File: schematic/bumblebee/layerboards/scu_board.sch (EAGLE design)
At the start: 19 parts, among them P5 B4B-EH-A, P7 B3B-EH-A, X1 332-02, X2 332-02, X3 332-02, X4 332-02, X5 332-02

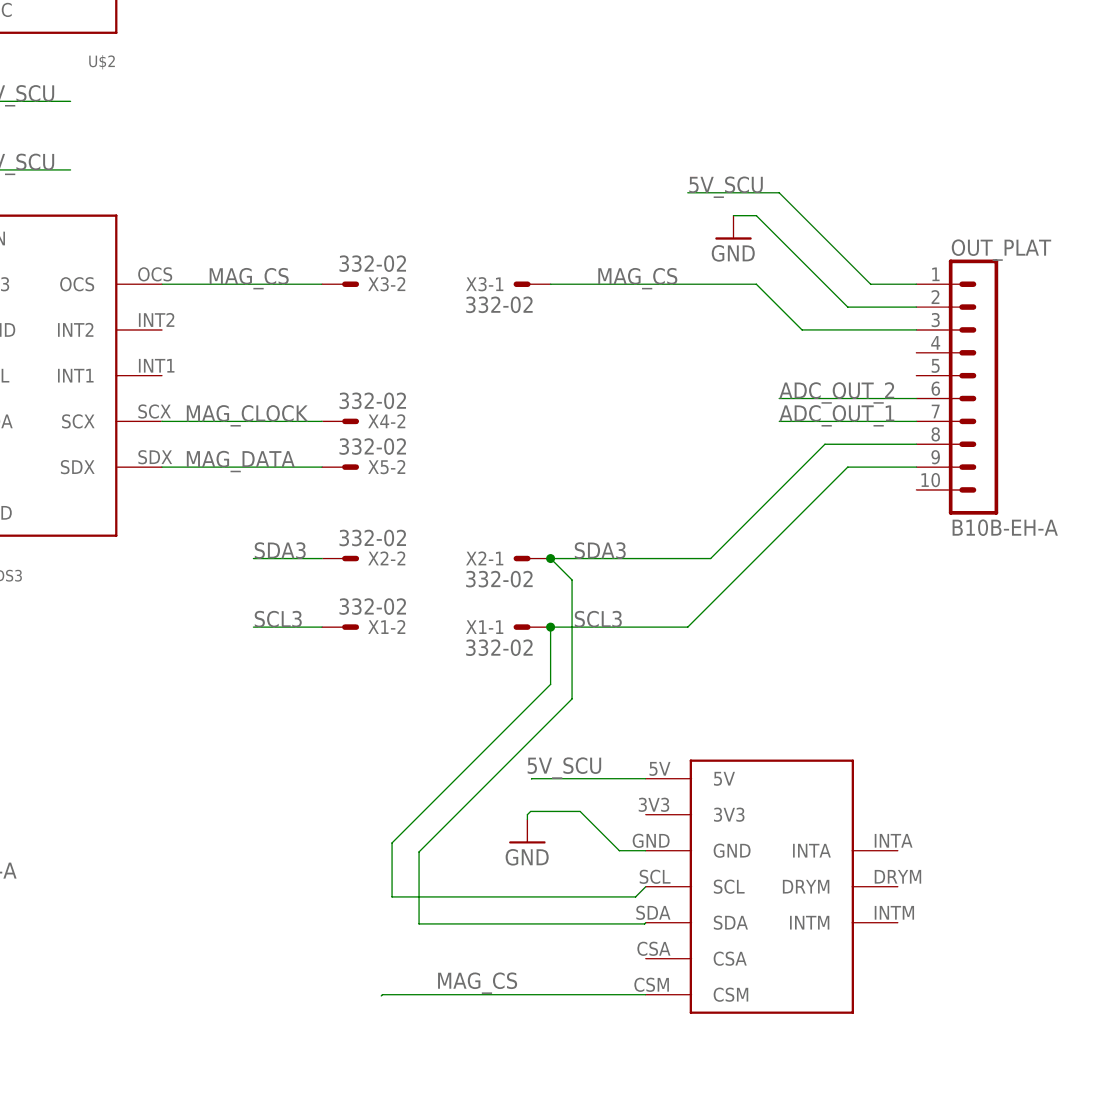
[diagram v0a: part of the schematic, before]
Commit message: Готова SCU и поправил lsm303c в либе
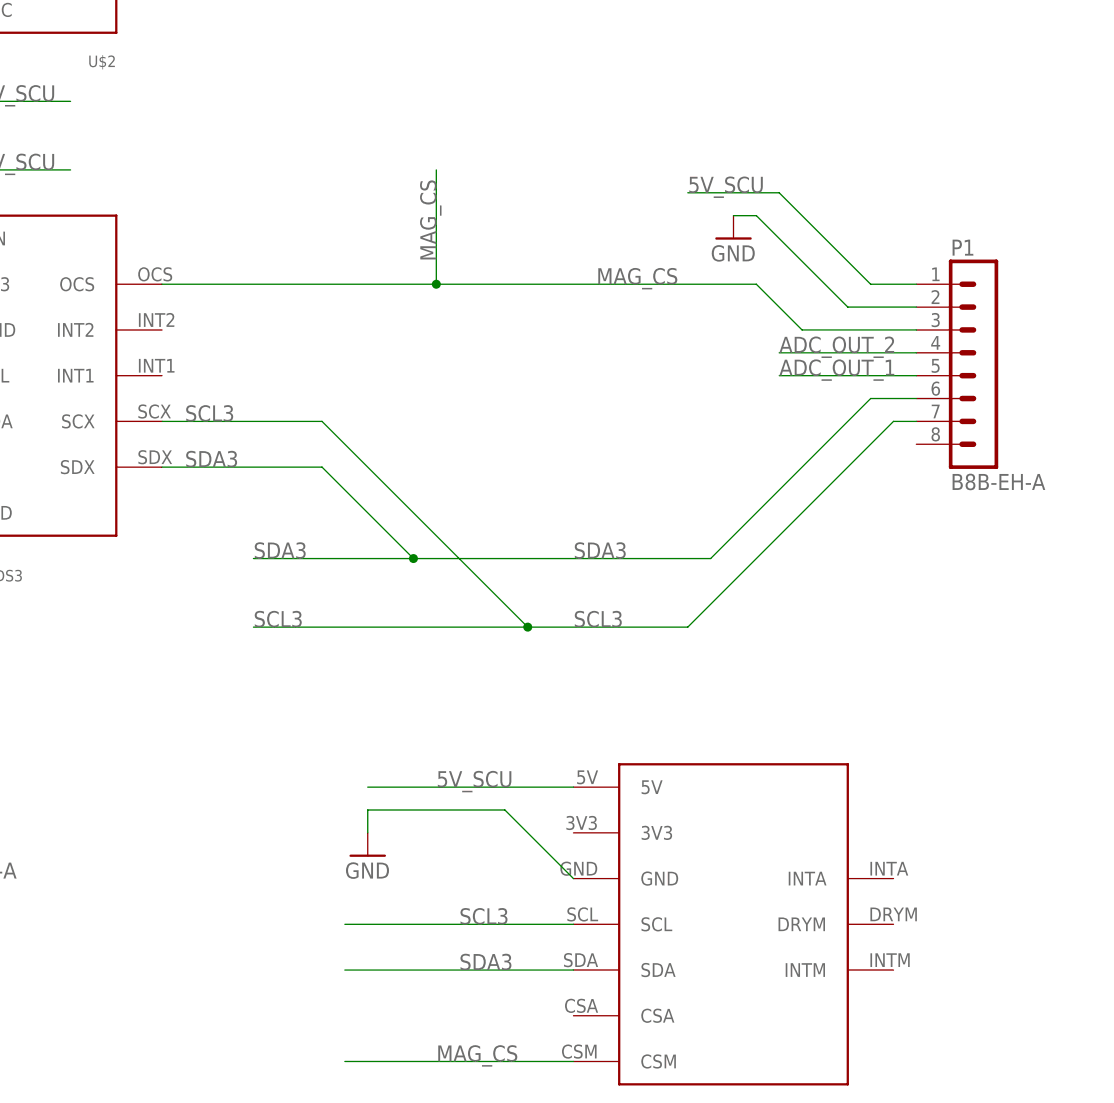
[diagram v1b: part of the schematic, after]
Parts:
- removed OUT_PLAT: B10B-EH-A, con-jst-eh:B10B-EH-A
- removed X1, X2, X3, X4, X5: 332-02, con-garry:332-02
- added P1: B8B-EH-A, con-jst-eh:B8B-EH-A
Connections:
- removed net MAG_CLOCK: U$3.SCX, X4-2.S
- removed net MAG_DATA: U$3.SDX, X5-2.S
- net 5V_SCU: now also P1.1; no longer OUT_PLAT.1
- net ADC_OUT_1: now also P1.5; no longer OUT_PLAT.7
- net ADC_OUT_2: now also P1.4; no longer OUT_PLAT.6
- net GND: now also P1.2; no longer OUT_PLAT.2
- net MAG_CS: now also P1.3; no longer OUT_PLAT.3, X3-1.S, X3-2.S
- net SCL3: now also P1.7, U$3.SCX; no longer OUT_PLAT.9, X1-1.S, X1-2.S
- net SDA3: now also P1.6, U$3.SDX; no longer OUT_PLAT.8, X2-1.S, X2-2.S
